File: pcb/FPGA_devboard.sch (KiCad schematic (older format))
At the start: 10 parts, among them X5 Conn_02x06_Odd_Even, X6 AC7020

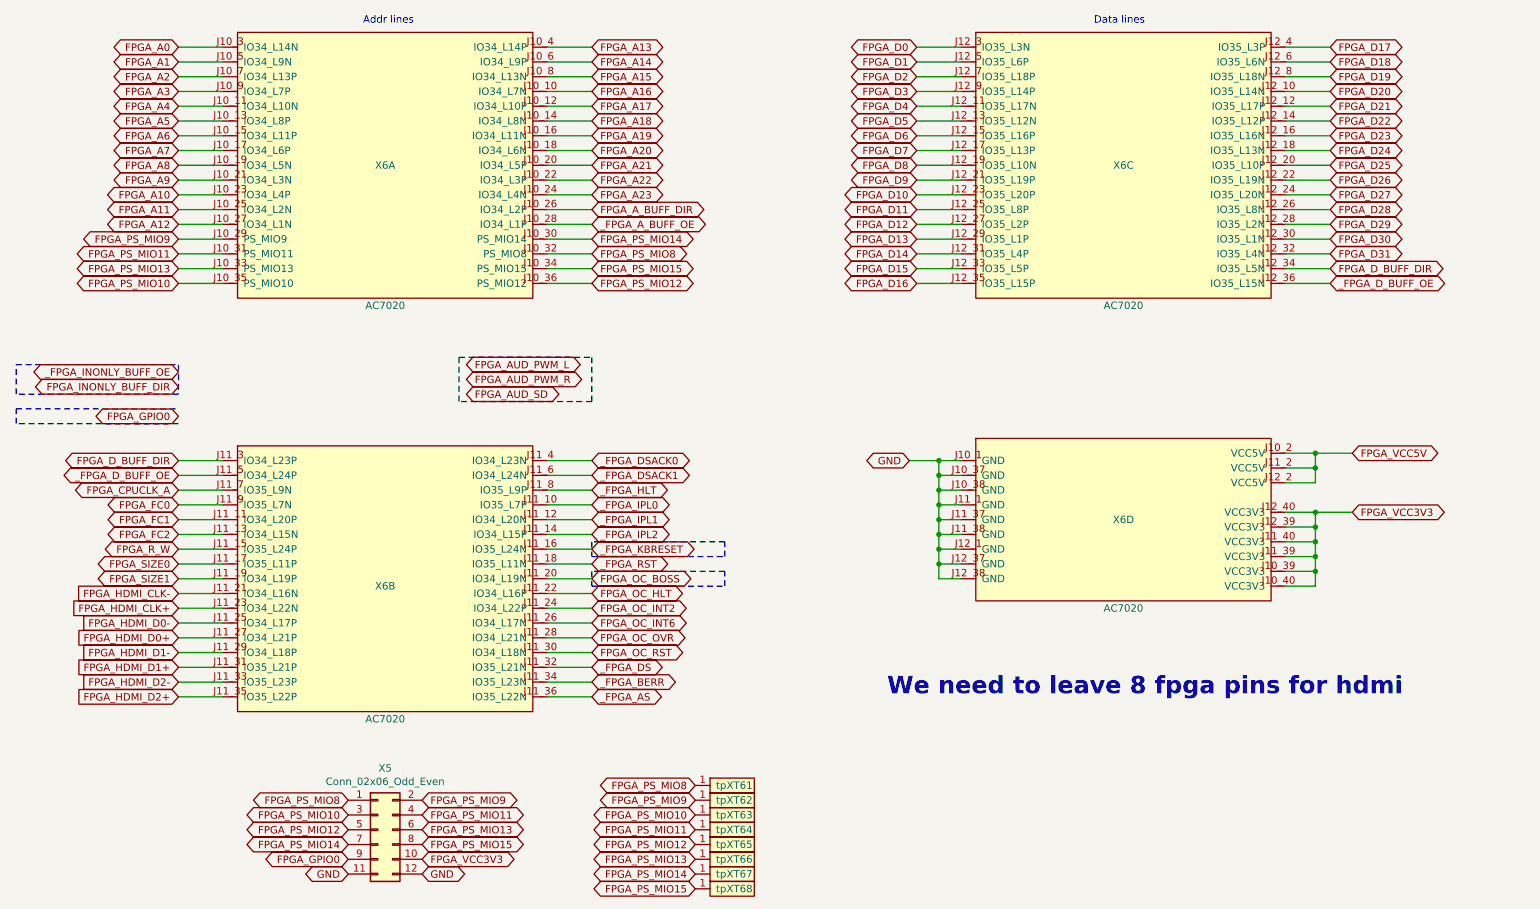
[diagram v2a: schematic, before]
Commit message: yet another wip commit
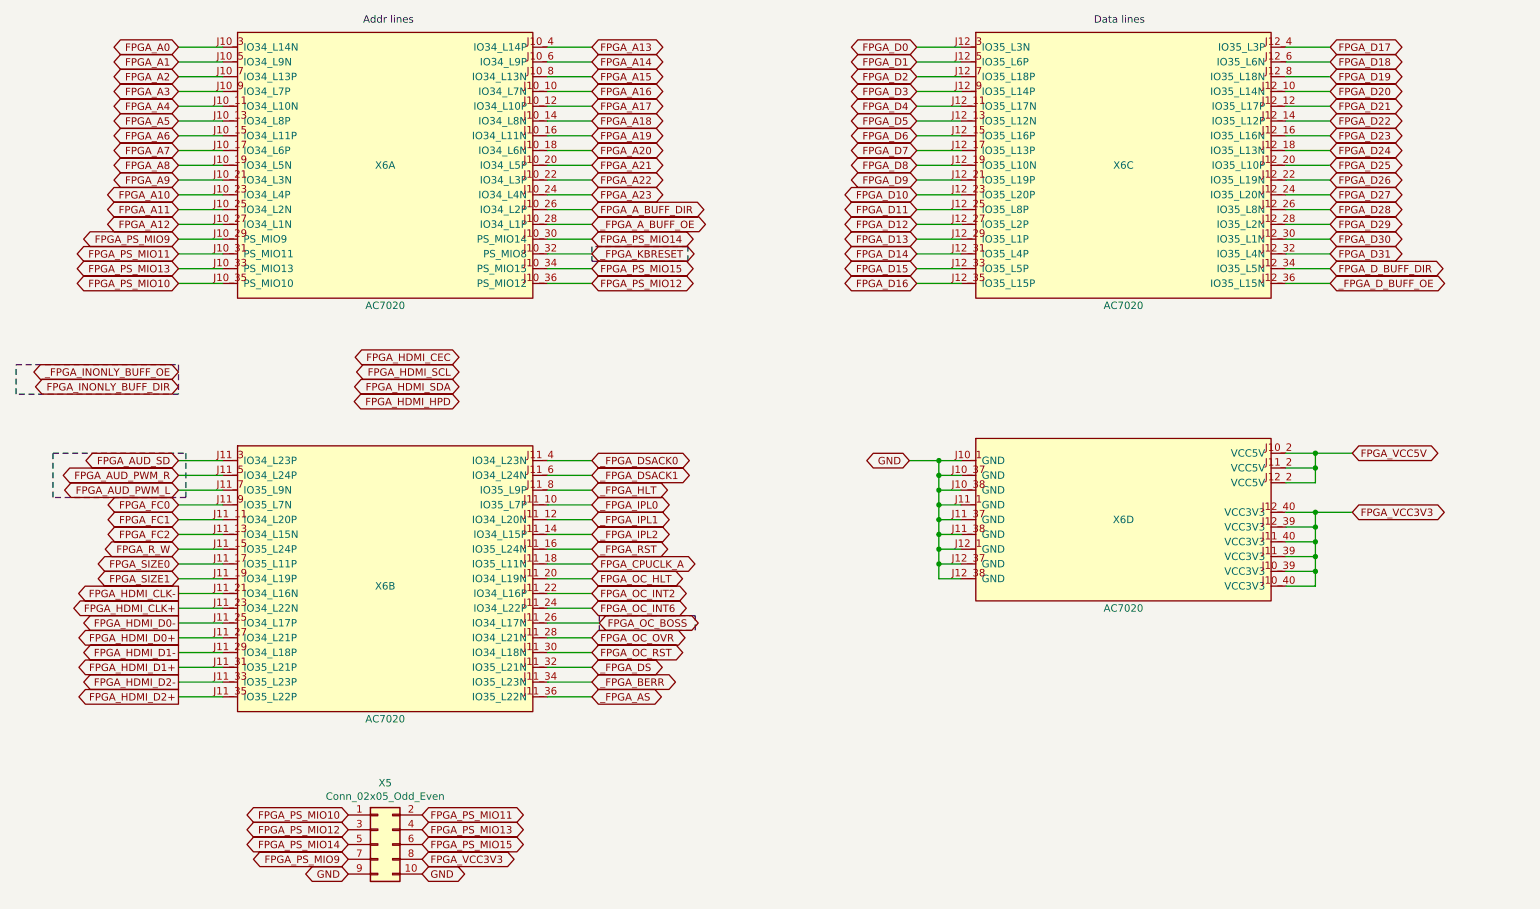
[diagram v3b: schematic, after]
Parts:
- removed X5: Conn_02x06_Odd_Even, symbol Connector_Generic:Conn_02x06_Odd_Even
- removed XT61, XT62, XT63, XT64, XT65, XT66, XT67, XT68: testpoint, symbol WM1200:testpoint
- added X5: Conn_02x05_Odd_Even, symbol Connector_Generic:Conn_02x05_Odd_Even
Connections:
- net FPGA_PS_MIO8 is gone; now on net _FPGA_KBRESET: X6.J10_32 (PS_MIO8)
- net FPGA_AUD_PWM_L: now also X6.J11_7 (IO35_L9N)
- net FPGA_AUD_PWM_R: now also X6.J11_5 (IO34_L24P)
- net FPGA_AUD_SD: now also X6.J11_3 (IO34_L23P)
- net FPGA_CPUCLK_A: now also X6.J11_18 (IO35_L11N); no longer X6.J11_7 (IO35_L9N)
- net FPGA_D_BUFF_DIR: no longer X6.J11_3 (IO34_L23P)
- net FPGA_OC_BOSS: now also X6.J11_26 (IO34_L17N); no longer X6.J11_20 (IO34_L19N)
- net FPGA_OC_HLT: now also X6.J11_20 (IO34_L19N); no longer X6.J11_22 (IO34_L16P)
- net FPGA_OC_INT2: now also X6.J11_22 (IO34_L16P); no longer X6.J11_24 (IO34_L22P)
- net FPGA_OC_INT6: now also X6.J11_24 (IO34_L22P); no longer X6.J11_26 (IO34_L17N)
- net FPGA_PS_MIO10: now also X5.1 (Pin_1)
- net FPGA_PS_MIO11: now also X5.2 (Pin_2)
- net FPGA_PS_MIO12: now also X5.3 (Pin_3)
- net FPGA_PS_MIO13: now also X5.4 (Pin_4)
- net FPGA_PS_MIO14: now also X5.5 (Pin_5)
- net FPGA_PS_MIO15: now also X5.6 (Pin_6)
- net FPGA_PS_MIO9: now also X5.7 (Pin_7)
- net FPGA_VCC3V3: now also X5.8 (Pin_8)
- net GND: now also X5.10 (Pin_10), X5.9 (Pin_9)
- net _FPGA_D_BUFF_OE: no longer X6.J11_5 (IO34_L24P)
- net _FPGA_KBRESET: no longer X6.J11_16 (IO35_L24N)
- net _FPGA_RST: now also X6.J11_16 (IO35_L24N); no longer X6.J11_18 (IO35_L11N)
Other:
- note removed: "We need to leave 8 fpga pins for hdmi"
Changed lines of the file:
@@
 	4300 2800 4600 2800
 Wire Wire Line
-	4300 4400 4600 4400
-Wire Wire Line
-	4600 4500 4300 4500
-Wire Wire Line
-	4300 4600 4600 4600
-Wire Wire Line
-	4600 4700 4300 4700
+	4300 5400 4600 5400
+Wire Wire Line
+	4600 4400 4300 4400
+Wire Wire Line
+	4300 4500 4600 4500
+Wire Wire Line
+	4600 4600 4300 4600
+Wire Wire Line
+	4300 4700 4600 4700
 Wire Wire Line
 	4300 4800 4600 4800
 Wire Wire Line
-	4300 4900 4600 4900
-Wire Wire Line
-	4300 5000 4600 5000
-Wire Wire Line
-	4600 5100 4300 5100
-Wire Wire Line
-	4300 5200 4600 5200
-Wire Wire Line
-	4600 5300 4300 5300
-Wire Wire Line
-	4300 5400 4600 5400
-Wire Wire Line
-	4600 5500 4300 5500
+	4600 5000 4300 5000
+Wire Wire Line
+	4600 5200 4300 5200
+Wire Wire Line
+	4300 5300 4600 5300
 Wire Wire Line
 	4300 5600 4600 5600
@@
 Text GLabel 9600 3200 2    50   BiDi ~ 0
 _FPGA_D_BUFF_OE
-Text GLabel 3750 3750 2    50   BiDi ~ 0
+Text GLabel 1800 4600 0    50   BiDi ~ 0
 FPGA_AUD_PWM_L
-Text GLabel 3750 3850 2    50   BiDi ~ 0
+Text GLabel 1800 4500 0    50   BiDi ~ 0
 FPGA_AUD_PWM_R
-Text GLabel 3750 3950 2    50   BiDi ~ 0
+Text GLabel 1800 4400 0    50   BiDi ~ 0
 FPGA_AUD_SD
+Text GLabel 4650 5500 2    50   BiDi ~ 0
+FPGA_OC_BOSS
 Text GLabel 4600 5200 2    50   BiDi ~ 0
-FPGA_OC_BOSS
-Text GLabel 4600 5300 2    50   BiDi ~ 0
 FPGA_OC_HLT
 Text GLabel 4600 5400 2    50   BiDi ~ 0
-FPGA_OC_INT2
-Text GLabel 4600 5500 2    50   BiDi ~ 0
 FPGA_OC_INT6
 Text GLabel 4600 5600 2    50   BiDi ~ 0
@@
 _FPGA_IPL2
 Text GLabel 4600 5000 2    50   BiDi ~ 0
-_FPGA_KBRESET
-Text GLabel 4600 5100 2    50   BiDi ~ 0
 _FPGA_RST
-$Comp
-L Connector_Generic:Conn_02x06_Odd_Even X5
-U 1 1 5E59EB5F
-P 3150 6900
-F 0 "X5" H 3200 7317 50  0000 C CNN
-F 1 "Conn_02x06_Odd_Even" H 3200 7226 50  0000 C CNN
-F 2 "" H 3150 6900 50  0001 C CNN
-F 3 "~" H 3150 6900 50  0001 C CNN
-	1    3150 6900
-	1    0    0    -1
-$EndComp
 Text GLabel 2950 7200 0    50   BiDi ~ 0
 GND
 Text GLabel 3450 7100 2    50   BiDi ~ 0
 FPGA_VCC3V3
-Text GLabel 1800 4100 0    50   BiDi ~ 0
-FPGA_GPIO0
-Text GLabel 2950 7100 0    50   BiDi ~ 0
-FPGA_GPIO0
-Text GLabel 1800 2900 0    50   BiDi ~ 0
-FPGA_PS_MIO9
 Text GLabel 1800 3000 0    50   BiDi ~ 0
 FPGA_PS_MIO11
@@
 Text GLabel 4600 3100 2    50   BiDi ~ 0
 FPGA_PS_MIO15
-Text GLabel 4600 3000 2    50   BiDi ~ 0
-FPGA_PS_MIO8
 Text GLabel 4600 2900 2    50   BiDi ~ 0
 FPGA_PS_MIO14
-Text GLabel 2950 6700 0    50   BiDi ~ 0
-FPGA_PS_MIO8
-Text GLabel 3450 6700 2    50   BiDi ~ 0
-FPGA_PS_MIO9
 Text GLabel 2950 6800 0    50   BiDi ~ 0
 FPGA_PS_MIO10
@@
 	1800 6000 2100 6000
 Wire Wire Line
-	1800 2900 2100 2900
-Wire Wire Line
 	2100 3000 1800 3000
 Wire Wire Line
@@
 	4300 2900 4600 2900
 Wire Wire Line
-	4600 3000 4300 3000
-Wire Wire Line
 	4300 3100 4600 3100
 Wire Wire Line
 	4600 3200 4300 3200
-$Comp
-L WM1200:testpoint XT61
-U 1 1 5E5A11BD
-P 5550 6650
-F 0 "XT61" H 5600 6700 50  0000 C CNN
-F 1 "testpoint" H 5550 6800 50  0001 C CNN
-F 2 "" H 5550 6650 50  0001 C CNN
-F 3 "" H 5550 6650 50  0001 C CNN
-	1    5550 6650
-	1    0    0    -1
-$EndComp
-$Comp
-L WM1200:testpoint XT62
-U 1 1 5E5B690A
-P 5550 6750
-F 0 "XT62" H 5600 6800 50  0000 C CNN
-F 1 "testpoint" H 5550 6900 50  0001 C CNN
-F 2 "" H 5550 6750 50  0001 C CNN
-F 3 "" H 5550 6750 50  0001 C CNN
-	1    5550 6750
-	1    0    0    -1
-$EndComp
-$Comp
-L WM1200:testpoint XT63
-U 1 1 5E5BE856
-P 5550 6850
-F 0 "XT63" H 5600 6900 50  0000 C CNN
-F 1 "testpoint" H 5550 7000 50  0001 C CNN
-F 2 "" H 5550 6850 50  0001 C CNN
-F 3 "" H 5550 6850 50  0001 C CNN
-	1    5550 6850
-	1    0    0    -1
-$EndComp
-$Comp
-L WM1200:testpoint XT64
-U 1 1 5E5C67D2
-P 5550 6950
-F 0 "XT64" H 5600 7000 50  0000 C CNN
-F 1 "testpoint" H 5550 7100 50  0001 C CNN
-F 2 "" H 5550 6950 50  0001 C CNN
-F 3 "" H 5550 6950 50  0001 C CNN
-	1    5550 6950
-	1    0    0    -1
-$EndComp
-$Comp
-L WM1200:testpoint XT65
-U 1 1 5E5CE745
-P 5550 7050
-F 0 "XT65" H 5600 7100 50  0000 C CNN
-F 1 "testpoint" H 5550 7200 50  0001 C CNN
-F 2 "" H 5550 7050 50  0001 C CNN
-F 3 "" H 5550 7050 50  0001 C CNN
-	1    5550 7050
-	1    0    0    -1
-$EndComp
-$Comp
-L WM1200:testpoint XT66
-U 1 1 5E5D6657
-P 5550 7150
-F 0 "XT66" H 5600 7200 50  0000 C CNN
-F 1 "testpoint" H 5550 7300 50  0001 C CNN
-F 2 "" H 5550 7150 50  0001 C CNN
-F 3 "" H 5550 7150 50  0001 C CNN
-	1    5550 7150
-	1    0    0    -1
-$EndComp
-$Comp
-L WM1200:testpoint XT67
-U 1 1 5E5DE64C
-P 5550 7250
-F 0 "XT67" H 5600 7300 50  0000 C CNN
-F 1 "testpoint" H 5550 7400 50  0001 C CNN
-F 2 "" H 5550 7250 50  0001 C CNN
-F 3 "" H 5550 7250 50  0001 C CNN
-	1    5550 7250
-	1    0    0    -1
-$EndComp
-$Comp
-L WM1200:testpoint XT68
-U 1 1 5E5E66B0
-P 5550 7350
-F 0 "XT68" H 5600 7400 50  0000 C CNN
-F 1 "testpoint" H 5550 7500 50  0001 C CNN
-F 2 "" H 5550 7350 50  0001 C CNN
-F 3 "" H 5550 7350 50  0001 C CNN
-	1    5550 7350
-	1    0    0    -1
-$EndComp
-Text GLabel 5300 6600 0    50   BiDi ~ 0
-FPGA_PS_MIO8
-Text GLabel 5300 6700 0    50   BiDi ~ 0
-FPGA_PS_MIO9
-Text GLabel 5300 6800 0    50   BiDi ~ 0
-FPGA_PS_MIO10
-Text GLabel 5300 6900 0    50   BiDi ~ 0
-FPGA_PS_MIO11
-Text GLabel 5300 7000 0    50   BiDi ~ 0
-FPGA_PS_MIO12
-Text GLabel 5300 7100 0    50   BiDi ~ 0
-FPGA_PS_MIO13
-Text GLabel 5300 7200 0    50   BiDi ~ 0
-FPGA_PS_MIO14
-Text GLabel 5300 7300 0    50   BiDi ~ 0
-FPGA_PS_MIO15
-Text Notes 6600 6000 0    118  ~ 24
-We need to leave 8 fpga pins for hdmi
-Wire Notes Line
-	4600 3700 4600 4000
-Wire Notes Line
-	4600 4000 3700 4000
-Wire Notes Line
-	3700 3700 4600 3700
-Wire Notes Line
-	5500 5150 4600 5150
-Wire Notes Line
-	4600 5150 4600 5250
-Wire Notes Line
-	4600 5250 5500 5250
-Wire Notes Line
-	5500 5250 5500 5150
+Wire Notes Line
+	950  4650 950  4350
+Wire Notes Line
+	950  4350 1850 4350
+Wire Notes Line
+	1850 4650 950  4650
+Wire Notes Line
+	5300 5450 4650 5450
+Wire Notes Line
+	4650 5450 4650 5550
+Wire Notes Line
+	4650 5550 5300 5550
+Wire Notes Line
+	5300 5550 5300 5450
 Wire Notes Line
 	1800 3750 1800 3950
@@
 	700  3950 700  3750
 Wire Notes Line
-	4600 4950 4600 5050
-Wire Notes Line
-	4600 5050 5500 5050
-Wire Notes Line
-	5500 5050 5500 4950
-Wire Notes Line
-	5500 4950 4600 4950
-Wire Notes Line
-	1800 4150 700  4150
-Wire Notes Line
-	700  4150 700  4050
-Wire Notes Line
-	700  4050 1800 4050
-Text GLabel 1800 6000 0    50   Input ~ 0
+	4600 3050 5250 3050
+Wire Notes Line
+	5250 3050 5250 2950
+Wire Notes Line
+	5250 2950 4600 2950
+Text GLabel 1800 6000 0    50   Output ~ 0
 FPGA_HDMI_D2+
-Text GLabel 1800 5900 0    50   Input ~ 0
+Text GLabel 1800 5900 0    50   Output ~ 0
 FPGA_HDMI_D2-
-Text GLabel 1800 5800 0    50   Input ~ 0
+Text GLabel 1800 5800 0    50   Output ~ 0
 FPGA_HDMI_D1+
-Text GLabel 1800 5600 0    50   Input ~ 0
+Text GLabel 1800 5600 0    50   Output ~ 0
 FPGA_HDMI_D0+
-Text GLabel 1800 5500 0    50   Input ~ 0
+Text GLabel 1800 5500 0    50   Output ~ 0
 FPGA_HDMI_D0-
-Text GLabel 1800 5700 0    50   Input ~ 0
+Text GLabel 1800 5700 0    50   Output ~ 0
 FPGA_HDMI_D1-
-Text GLabel 1800 5400 0    50   Input ~ 0
+Text GLabel 1800 5400 0    50   Output ~ 0
 FPGA_HDMI_CLK+
-Text GLabel 1800 5300 0    50   Input ~ 0
-FPGA_HDMI_CLK-
 Wire Notes Line
 	1800 3950 700  3950
@@
 Text GLabel 1800 4700 0    50   BiDi ~ 0
 FPGA_FC0
-Text GLabel 1800 4600 0    50   BiDi ~ 0
+Text GLabel 4600 5100 2    50   BiDi ~ 0
 FPGA_CPUCLK_A
 Text GLabel 1800 3900 0    50   BiDi ~ 0
@@
 Text GLabel 1800 3800 0    50   BiDi ~ 0
 _FPGA_INONLY_BUFF_OE
-Text GLabel 1800 4400 0    50   BiDi ~ 0
-FPGA_D_BUFF_DIR
-Text GLabel 1800 4500 0    50   BiDi ~ 0
-_FPGA_D_BUFF_OE
-Wire Notes Line
-	3700 4000 3700 3700
+Wire Notes Line
+	1850 4350 1850 4650
+Text GLabel 1800 5300 0    50   Output ~ 0
+FPGA_HDMI_CLK-
+Wire Wire Line
+	1800 2900 2100 2900
+Text GLabel 4600 3000 2    50   BiDi ~ 0
+_FPGA_KBRESET
+Wire Notes Line
+	4600 2950 4600 3050
+Wire Wire Line
+	4600 4900 4300 4900
+Wire Wire Line
+	4300 5100 4600 5100
+$Comp
+L Connector_Generic:Conn_02x05_Odd_Even X5
+U 1 1 5E864C32
+P 3150 7000
+F 0 "X5" H 3200 7417 50  0000 C CNN
+F 1 "Conn_02x05_Odd_Even" H 3200 7326 50  0000 C CNN
+F 2 "" H 3150 7000 50  0001 C CNN
+F 3 "~" H 3150 7000 50  0001 C CNN
+	1    3150 7000
+	1    0    0    -1
+$EndComp
+Text GLabel 3700 3700 0    50   BiDi ~ 0
+FPGA_HDMI_CEC
+Text GLabel 3700 3800 0    50   BiDi ~ 0
+FPGA_HDMI_SCL
+Text GLabel 3700 3900 0    50   BiDi ~ 0
+FPGA_HDMI_SDA
+Text GLabel 3700 4000 0    50   BiDi ~ 0
+FPGA_HDMI_HPD
+Text GLabel 4600 5300 2    50   BiDi ~ 0
+FPGA_OC_INT2
+Wire Wire Line
+	4300 5500 4650 5500
+Text GLabel 2950 7100 0    50   BiDi ~ 0
+FPGA_PS_MIO9
+Text GLabel 1800 2900 0    50   BiDi ~ 0
+FPGA_PS_MIO9
+Wire Wire Line
+	4300 3000 4600 3000
 $EndSCHEMATC
